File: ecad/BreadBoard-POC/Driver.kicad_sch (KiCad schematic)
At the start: 24 parts, among them J1 Conn_01x01, J2 Conn_01x01, J3 Conn_01x01, J4 Conn_01x01, U1 L6205N

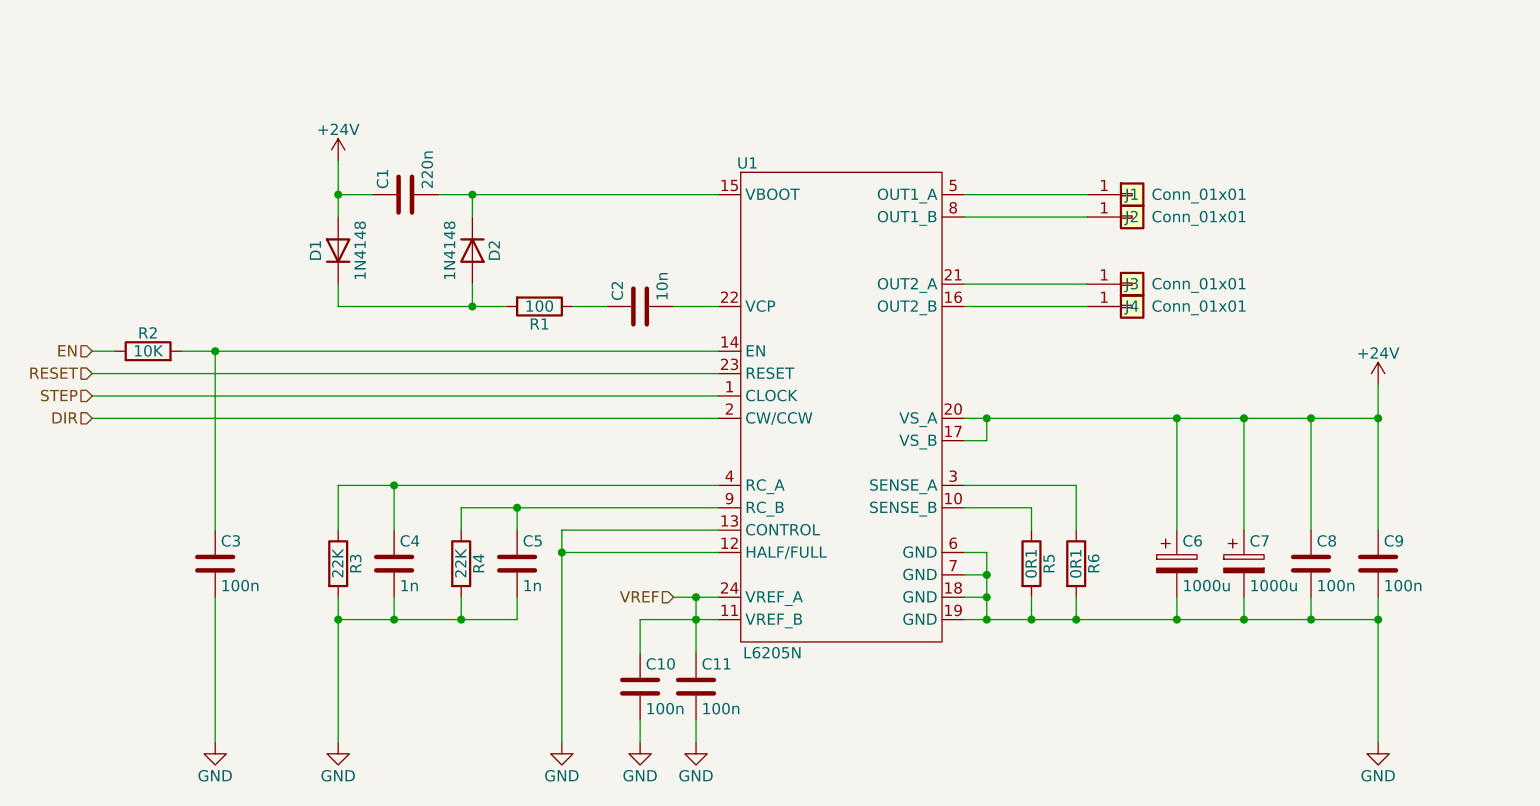
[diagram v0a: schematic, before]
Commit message: Finalizing POC placement and routing.
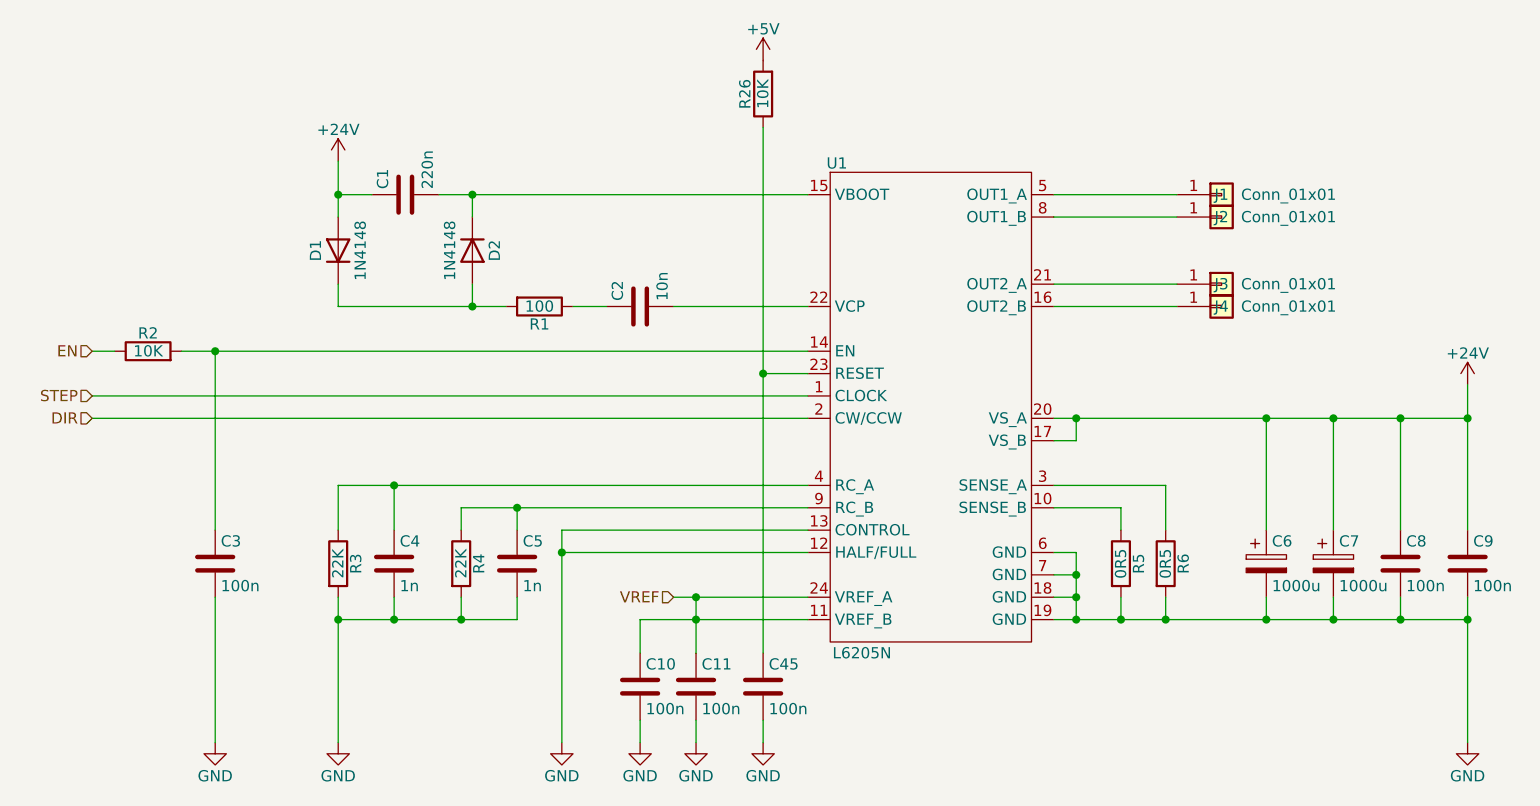
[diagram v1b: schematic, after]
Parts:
- added C45: 100n, Capacitor_THT:C_Rect_L4.6mm_W2.0mm_P2.50mm_MKS02_FKP02, symbol Device:C
- added R26: 10K, Resistor_THT:R_Axial_DIN0207_L6.3mm_D2.5mm_P2.54mm_Vertical, symbol Device:R
- R5, R6: value 0R1 -> 0R5
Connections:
- net GND: now also C45.2
- net RESET: no longer names the net of U1.23 (RESET)
- net RESET: now also C45.1, R26.1
- new net +5V: R26.2
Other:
- moved on the sheet: C6, C7, C8, C9, J1, J2, J3, J4, R5, R6, U1
